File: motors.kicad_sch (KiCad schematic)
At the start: 6 parts, among them J3 Conn_01x02, J4 Conn_01x02, J5 Conn_01x02, J6 Conn_01x02, U5 TB6612FNG, U6 TB6612FNG

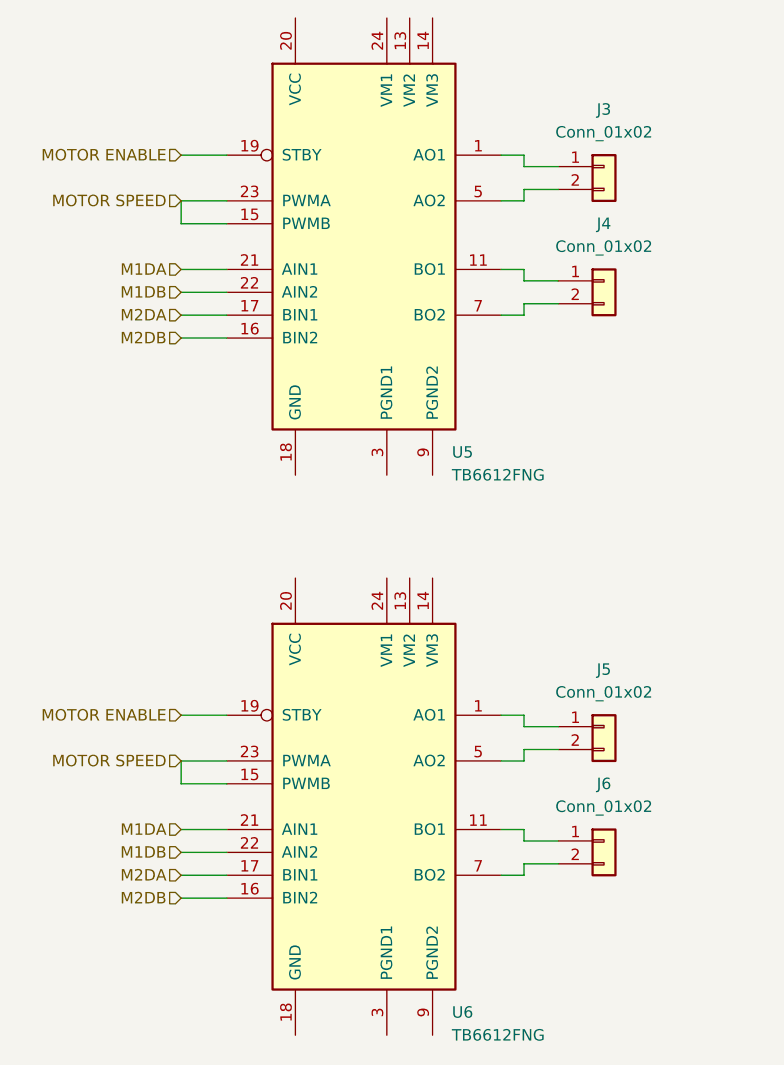
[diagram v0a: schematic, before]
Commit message: feat: nets and stuff?? I guess?
I don't really remember what this commit changes
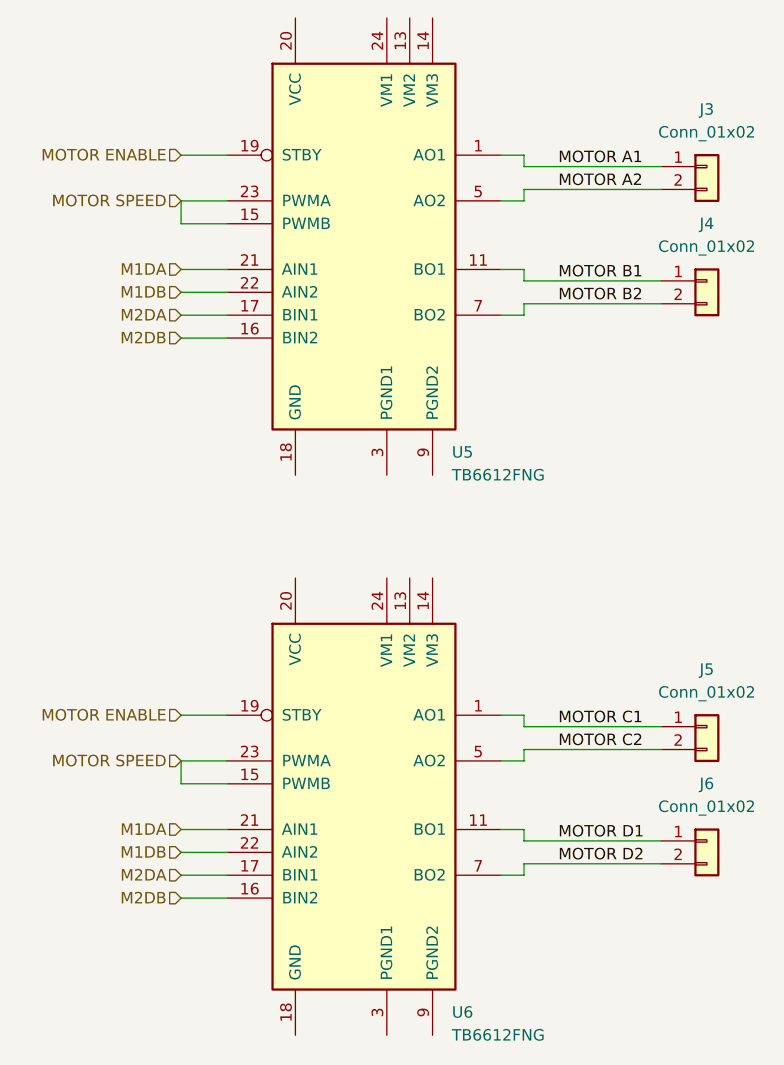
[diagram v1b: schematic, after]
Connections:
- net MOTOR B1: now reaches J4.1 (Pin_1), U5.11 (BO1), U5.12 (BO1)
- net MOTOR B2: now reaches J4.2 (Pin_2), U5.7 (BO2), U5.8 (BO2)
- net MOTOR C1: now reaches J5.1 (Pin_1), U6.1 (AO1), U6.2 (AO1)
- net MOTOR D1: now reaches J6.1 (Pin_1), U6.11 (BO1), U6.12 (BO1)
- net MOTOR C2: now reaches J5.2 (Pin_2), U6.5 (AO2), U6.6 (AO2)
- net MOTOR D2: now reaches J6.2 (Pin_2), U6.7 (BO2), U6.8 (BO2)
- net MOTOR A1: now reaches J3.1 (Pin_1), U5.1 (AO1), U5.2 (AO1)
- net MOTOR A2: now reaches J3.2 (Pin_2), U5.5 (AO2), U5.6 (AO2)
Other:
- moved on the sheet: J3, J4, J5, J6
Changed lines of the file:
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@@
 	(wire
 		(pts
-			(xy 152.4 139.7) (xy 148.59 139.7)
+			(xy 163.83 139.7) (xy 148.59 139.7)
 		)
 		(stroke
@@
 	(wire
 		(pts
-			(xy 152.4 127) (xy 148.59 127)
+			(xy 163.83 127) (xy 148.59 127)
 		)
 		(stroke
@@
 	(wire
 		(pts
-			(xy 152.4 77.47) (xy 148.59 77.47)
+			(xy 163.83 77.47) (xy 148.59 77.47)
 		)
 		(stroke
@@
 	(wire
 		(pts
-			(xy 148.59 62.23) (xy 152.4 62.23)
-		)
-		(stroke
-			(width 0)
-			(type default)
-		)
-	)
-	(wire
-		(pts
-			(xy 148.59 135.89) (xy 148.59 137.16)
+			(xy 148.59 62.23) (xy 163.83 62.23)
+		)
+		(stroke
+			(width 0)
+			(type default)
+		)
+	)
+	(wire
+		(pts
+			(xy 148.59 137.16) (xy 148.59 135.89)
 		)
 		(stroke
@@
 	(wire
 		(pts
-			(xy 148.59 124.46) (xy 152.4 124.46)
+			(xy 148.59 124.46) (xy 163.83 124.46)
 		)
 		(stroke
@@
 	(wire
 		(pts
-			(xy 148.59 73.66) (xy 148.59 74.93)
+			(xy 148.59 74.93) (xy 148.59 73.66)
 		)
 		(stroke
@@
 	(wire
 		(pts
-			(xy 152.4 64.77) (xy 148.59 64.77)
+			(xy 163.83 64.77) (xy 148.59 64.77)
 		)
 		(stroke
@@
 	(wire
 		(pts
-			(xy 148.59 74.93) (xy 152.4 74.93)
+			(xy 148.59 74.93) (xy 163.83 74.93)
 		)
 		(stroke
@@
 	(wire
 		(pts
-			(xy 148.59 123.19) (xy 148.59 124.46)
-		)
-		(stroke
-			(width 0)
-			(type default)
-		)
-	)
-	(wire
-		(pts
-			(xy 148.59 137.16) (xy 152.4 137.16)
-		)
-		(stroke
-			(width 0)
-			(type default)
+			(xy 148.59 124.46) (xy 148.59 123.19)
+		)
+		(stroke
+			(width 0)
+			(type default)
+		)
+	)
+	(wire
+		(pts
+			(xy 148.59 137.16) (xy 163.83 137.16)
+		)
+		(stroke
+			(width 0)
+			(type default)
+		)
+	)
+	(label "MOTOR B1"
+		(at 152.4 74.93 0)
+		(effects
+			(font
+				(size 1.27 1.27)
+			)
+			(justify left bottom)
+		)
+	)
+	(label "MOTOR D1"
+		(at 152.4 137.16 0)
+		(effects
+			(font
+				(size 1.27 1.27)
+			)
+			(justify left bottom)
+		)
+	)
+	(label "MOTOR C2"
+		(at 152.4 127 0)
+		(effects
+			(font
+				(size 1.27 1.27)
+			)
+			(justify left bottom)
+		)
+	)
+	(label "MOTOR C1"
+		(at 152.4 124.46 0)
+		(effects
+			(font
+				(size 1.27 1.27)
+			)
+			(justify left bottom)
+		)
+	)
+	(label "MOTOR A1"
+		(at 152.4 62.23 0)
+		(effects
+			(font
+				(size 1.27 1.27)
+			)
+			(justify left bottom)
+		)
+	)
+	(label "MOTOR B2"
+		(at 152.4 77.47 0)
+		(effects
+			(font
+				(size 1.27 1.27)
+			)
+			(justify left bottom)
+		)
+	)
+	(label "MOTOR D2"
+		(at 152.4 139.7 0)
+		(effects
+			(font
+				(size 1.27 1.27)
+			)
+			(justify left bottom)
+		)
+	)
+	(label "MOTOR A2"
+		(at 152.4 64.77 0)
+		(effects
+			(font
+				(size 1.27 1.27)
+			)
+			(justify left bottom)
 		)
 	)
@@
 	(symbol
 		(lib_id "Connector_Generic:Conn_01x02")
-		(at 157.48 74.93 0)
+		(at 168.91 74.93 0)
 		(unit 1)
 		(exclude_from_sim no)
@@
 		(dnp no)
 		(property "Reference" "J4"
-			(at 157.48 68.58 0)
+			(at 168.91 68.58 0)
 			(effects
 				(font
@@
 		)
 		(property "Value" "Conn_01x02"
-			(at 157.48 71.12 0)
+			(at 168.91 71.12 0)
 			(effects
 				(font
@@
 		)
 		(property "Footprint" "Connector_PinHeader_2.54mm:PinHeader_1x02_P2.54mm_Vertical"
-			(at 157.48 74.93 0)
+			(at 168.91 74.93 0)
 			(effects
 				(font
@@
 		)
 		(property "Datasheet" "~"
-			(at 157.48 74.93 0)
+			(at 168.91 74.93 0)
 			(effects
 				(font
@@
 		)
 		(property "Description" "Generic connector, single row, 01x02, script generated (kicad-library-utils/schlib/autogen/connector/)"
-			(at 157.48 74.93 0)
+			(at 168.91 74.93 0)
 			(effects
 				(font
@@
 	(symbol
 		(lib_id "Connector_Generic:Conn_01x02")
-		(at 157.48 62.23 0)
+		(at 168.91 62.23 0)
 		(unit 1)
 		(exclude_from_sim no)
@@
 		(dnp no)
 		(property "Reference" "J3"
-			(at 157.48 55.88 0)
+			(at 168.91 55.88 0)
 			(effects
 				(font
@@
 		)
 		(property "Value" "Conn_01x02"
-			(at 157.48 58.42 0)
+			(at 168.91 58.42 0)
 			(effects
 				(font
@@
 		)
 		(property "Footprint" "Connector_PinHeader_2.54mm:PinHeader_1x02_P2.54mm_Vertical"
-			(at 157.48 62.23 0)
+			(at 168.91 62.23 0)
 			(effects
 				(font
@@
 		)
 		(property "Datasheet" "~"
-			(at 157.48 62.23 0)
+			(at 168.91 62.23 0)
 			(effects
 				(font
@@
 		)
 		(property "Description" "Generic connector, single row, 01x02, script generated (kicad-library-utils/schlib/autogen/connector/)"
-			(at 157.48 62.23 0)
+			(at 168.91 62.23 0)
 			(effects
 				(font
@@
 	(symbol
 		(lib_id "Connector_Generic:Conn_01x02")
-		(at 157.48 137.16 0)
+		(at 168.91 137.16 0)
 		(unit 1)
 		(exclude_from_sim no)
@@
 		(dnp no)
 		(property "Reference" "J6"
-			(at 157.48 130.81 0)
+			(at 168.91 130.81 0)
 			(effects
 				(font
@@
 		)
 		(property "Value" "Conn_01x02"
-			(at 157.48 133.35 0)
+			(at 168.91 133.35 0)
 			(effects
 				(font
@@
 		)
 		(property "Footprint" "Connector_PinHeader_2.54mm:PinHeader_1x02_P2.54mm_Vertical"
-			(at 157.48 137.16 0)
+			(at 168.91 137.16 0)
 			(effects
 				(font
@@
 		)
 		(property "Datasheet" "~"
-			(at 157.48 137.16 0)
+			(at 168.91 137.16 0)
 			(effects
 				(font
@@
 		)
 		(property "Description" "Generic connector, single row, 01x02, script generated (kicad-library-utils/schlib/autogen/connector/)"
-			(at 157.48 137.16 0)
+			(at 168.91 137.16 0)
 			(effects
 				(font
@@
 	(symbol
 		(lib_id "Connector_Generic:Conn_01x02")
-		(at 157.48 124.46 0)
+		(at 168.91 124.46 0)
 		(unit 1)
 		(exclude_from_sim no)
@@
 		(dnp no)
 		(property "Reference" "J5"
-			(at 157.48 118.11 0)
+			(at 168.91 118.11 0)
 			(effects
 				(font
@@
 		)
 		(property "Value" "Conn_01x02"
-			(at 157.48 120.65 0)
+			(at 168.91 120.65 0)
 			(effects
 				(font
@@
 		)
 		(property "Footprint" "Connector_PinHeader_2.54mm:PinHeader_1x02_P2.54mm_Vertical"
-			(at 157.48 124.46 0)
+			(at 168.91 124.46 0)
 			(effects
 				(font
@@
 		)
 		(property "Datasheet" "~"
-			(at 157.48 124.46 0)
+			(at 168.91 124.46 0)
 			(effects
 				(font
@@
 		)
 		(property "Description" "Generic connector, single row, 01x02, script generated (kicad-library-utils/schlib/autogen/connector/)"
-			(at 157.48 124.46 0)
-			(effects
-				(font
+			(at 168.91 124.46 0)
+			(effects
+				(font
